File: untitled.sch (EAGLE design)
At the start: 2 parts

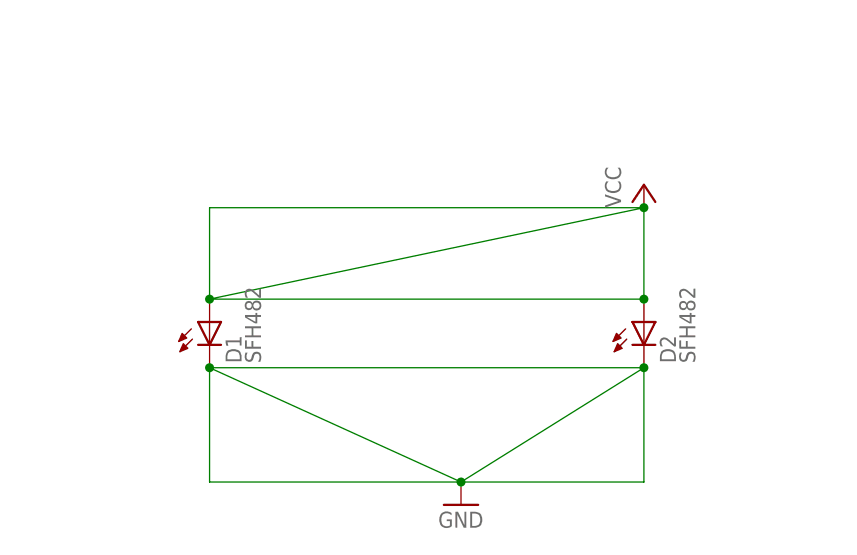
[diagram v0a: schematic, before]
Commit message: Add files via upload
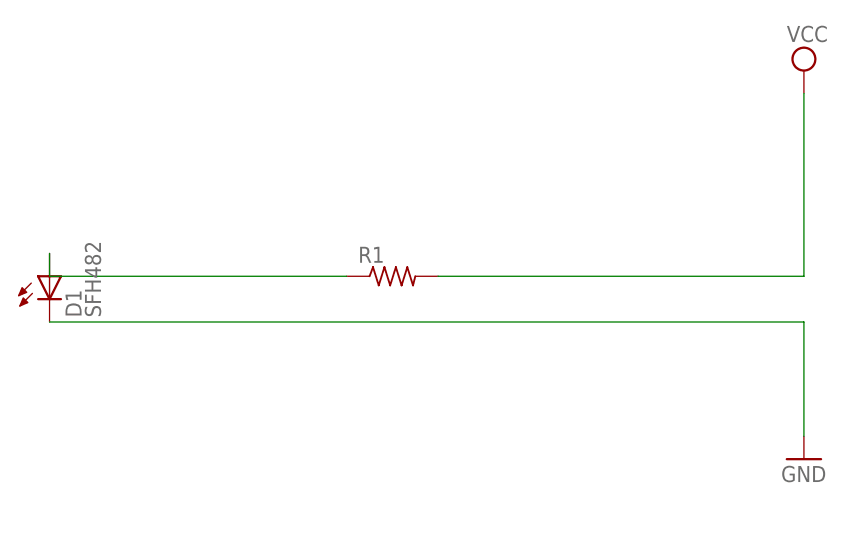
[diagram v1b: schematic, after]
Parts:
- removed D2: SFH482, led:SFH482
- added R1: (no value), resistor:R-US_0204/2V
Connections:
- new net N$1: D1.A, R1.1
- net GND: no longer D2.C
- net VCC: now also R1.2; no longer D1.A, D2.A
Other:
- moved on the sheet: D1
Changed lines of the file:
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@@
 <layer number="40" name="bKeepout" color="1" fill="11" visible="no" active="no"/>
 <layer number="41" name="tRestrict" color="4" fill="10" visible="no" active="no"/>
-<layer number="42" name="bRestrict" color="1" fill="10" visible="no" active="no"/>
+<layer number="42" name="bRestrict" color="3" fill="10" visible="no" active="no"/>
 <layer number="43" name="vRestrict" color="2" fill="10" visible="no" active="no"/>
 <layer number="44" name="Drills" color="7" fill="1" visible="no" active="no"/>
@@
 <layer number="97" name="Info" color="7" fill="1" visible="yes" active="yes"/>
 <layer number="98" name="Guide" color="6" fill="1" visible="yes" active="yes"/>
+<layer number="99" name="SpiceOrder" color="5" fill="1" visible="yes" active="yes"/>
 </layers>
 <schematic xreflabel="%F%N/%S.%C%R" xrefpart="/%S.%C%R">
@@
 </classes>
 <parts>
+<part name="SUPPLY1" library="supply2" library_urn="urn:adsk.eagle:library:372" deviceset="VCC" device=""/>
 <part name="GND1" library="supply1" library_urn="urn:adsk.eagle:library:371" deviceset="GND" device=""/>
-<part name="P+1" library="supply1" library_urn="urn:adsk.eagle:library:371" deviceset="VCC" device=""/>
+<part name="R1" library="resistor" library_urn="urn:adsk.eagle:library:348" deviceset="R-US_" device="0204/2V" package3d_urn="urn:adsk.eagle:package:25948/1"/>
 <part name="D1" library="led" library_urn="urn:adsk.eagle:library:259" deviceset="SFH482" device="" package3d_urn="urn:adsk.eagle:package:15795/1"/>
-<part name="D2" library="led" library_urn="urn:adsk.eagle:library:259" deviceset="SFH482" device="" package3d_urn="urn:adsk.eagle:package:15795/1"/>
 </parts>
 <sheets>
@@
 </plain>
 <instances>
-<instance part="GND1" gate="1" x="66.04" y="43.18"/>
-<instance part="P+1" gate="VCC" x="86.36" y="78.74"/>
-<instance part="D1" gate="1" x="38.1" y="63.5"/>
-<instance part="D2" gate="1" x="86.36" y="63.5"/>
+<instance part="SUPPLY1" gate="G$1" x="104.14" y="91.44"/>
+<instance part="GND1" gate="1" x="104.14" y="48.26"/>
+<instance part="R1" gate="G$1" x="58.42" y="68.58"/>
+<instance part="D1" gate="1" x="20.32" y="68.58"/>
 </instances>
 <busses>
@@
 <net name="VCC" class="0">
 <segment>
-<pinref part="P+1" gate="VCC" pin="VCC"/>
+<pinref part="SUPPLY1" gate="G$1" pin="VCC"/>
+<pinref part="R1" gate="G$1" pin="2"/>
+<wire x1="104.14" y1="88.9" x2="104.14" y2="68.58" width="0.1524" layer="91"/>
+<wire x1="104.14" y1="68.58" x2="63.5" y2="68.58" width="0.1524" layer="91"/>
+</segment>
+</net>
+<net name="N$1" class="0">
+<segment>
+<pinref part="R1" gate="G$1" pin="1"/>
 <pinref part="D1" gate="1" pin="A"/>
-<wire x1="86.36" y1="76.2" x2="38.1" y2="76.2" width="0.1524" layer="91"/>
-<wire x1="38.1" y1="76.2" x2="38.1" y2="66.04" width="0.1524" layer="91"/>
-<wire x1="86.36" y1="76.2" x2="38.1" y2="66.04" width="0.1524" layer="91"/>
-<junction x="86.36" y="76.2"/>
-<junction x="38.1" y="66.04"/>
-<pinref part="D2" gate="1" pin="A"/>
-<wire x1="38.1" y1="66.04" x2="86.36" y2="66.04" width="0.1524" layer="91"/>
-<wire x1="86.36" y1="76.2" x2="86.36" y2="66.04" width="0.1524" layer="91"/>
-<junction x="86.36" y="66.04"/>
+<wire x1="53.34" y1="68.58" x2="20.32" y2="68.58" width="0.1524" layer="91"/>
+<wire x1="20.32" y1="68.58" x2="20.32" y2="71.12" width="0.1524" layer="91"/>
 </segment>
 </net>
@@
 <pinref part="D1" gate="1" pin="C"/>
 <pinref part="GND1" gate="1" pin="GND"/>
-<wire x1="38.1" y1="58.42" x2="38.1" y2="45.72" width="0.1524" layer="91"/>
-<wire x1="38.1" y1="45.72" x2="66.04" y2="45.72" width="0.1524" layer="91"/>
-<wire x1="38.1" y1="58.42" x2="66.04" y2="45.72" width="0.1524" layer="91"/>
-<junction x="38.1" y="58.42"/>
-<junction x="66.04" y="45.72"/>
-<pinref part="D2" gate="1" pin="C"/>
-<wire x1="38.1" y1="58.42" x2="86.36" y2="58.42" width="0.1524" layer="91"/>
-<wire x1="86.36" y1="58.42" x2="66.04" y2="45.72" width="0.1524" layer="91"/>
-<junction x="86.36" y="58.42"/>
-<wire x1="86.36" y1="58.42" x2="86.36" y2="45.72" width="0.1524" layer="91"/>
-<wire x1="86.36" y1="45.72" x2="66.04" y2="45.72" width="0.1524" layer="91"/>
+<wire x1="20.32" y1="63.5" x2="104.14" y2="63.5" width="0.1524" layer="91"/>
+<wire x1="104.14" y1="63.5" x2="104.14" y2="50.8" width="0.1524" layer="91"/>
 </segment>
 </net>
